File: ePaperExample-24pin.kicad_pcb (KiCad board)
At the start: 2 copper layers, 20 parts, among them J1 Conn_01x24_MountingPin, Q1 Q_NMOS_GSD

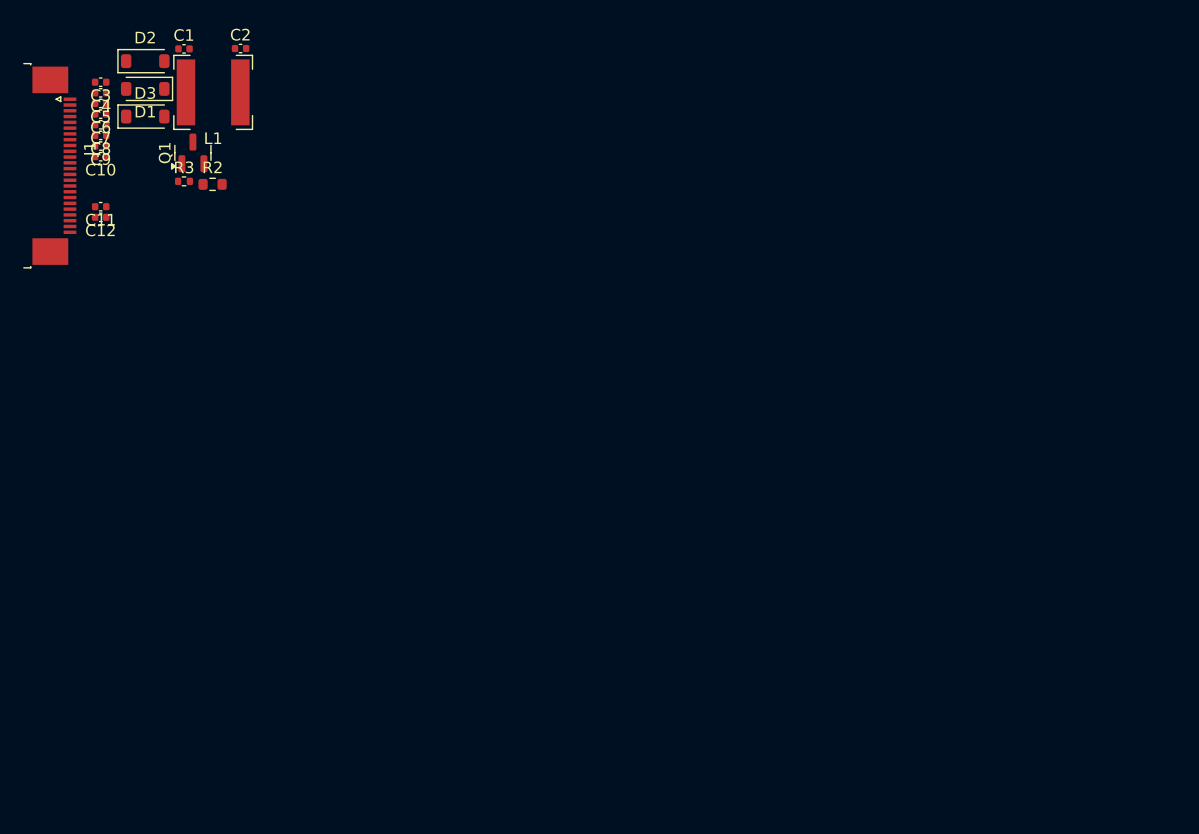
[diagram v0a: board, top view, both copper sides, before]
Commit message: Added updated schematic, added PCB layout
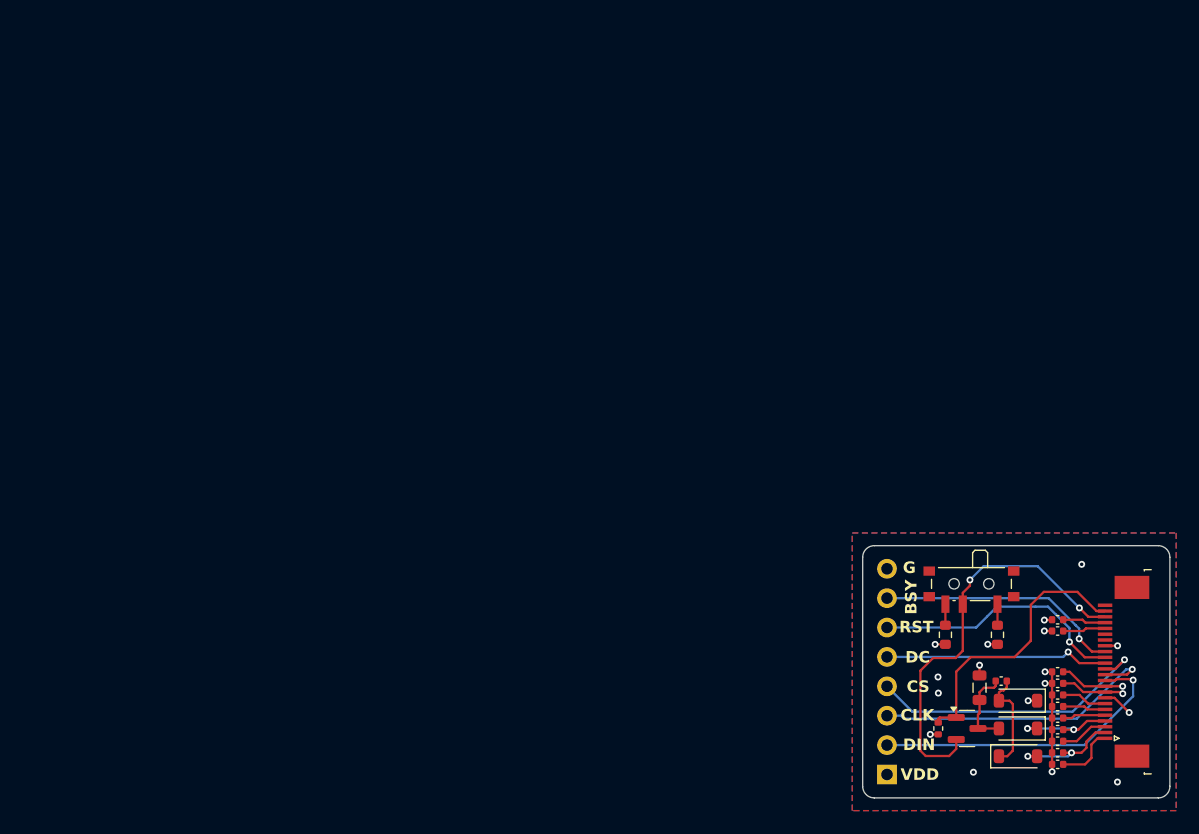
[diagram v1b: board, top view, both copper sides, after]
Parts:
- added J2: Conn_01x08_Socket, Connector_PinHeader_2.54mm:PinHeader_1x08_P2.54mm_Vertical, B.Cu at (129.0, 111.5)
- added R1: 1MR, Resistor_SMD:R_0402_1005Metric, F.Cu at (133.4, 107.5)
- added SW1: SW_SPDT, Button_Switch_SMD:SW_SPDT_PCM12, F.Cu at (136.3, 95.3)
- C1: value 100nF -> 1uF
- C2: value 4.7uF -> 1uF
- C4, C9: value 1uF -> 4.7uF
- L1: value 68uH -> 10uH; footprint Inductor_SMD:L_Bourns-SRN6028 -> Inductor_SMD:L_0805_2012Metric
- R2: value 3R -> 0R47
- R3: value 1MR -> 3R; footprint Resistor_SMD:R_0402_1005Metric -> Resistor_SMD:R_0603_1608Metric
- moved J1 102.0 mm to (149.2, 102.6), turned to 90 degrees
- moved C3 100.4 mm to (143.8, 108.6), turned to 0 degrees
- moved C5 98.8 mm to (143.8, 107.6), turned to 0 degrees
- moved C6 97.8 mm to (143.8, 106.6), turned to 0 degrees
- moved C1 97.6 mm to (143.8, 110.6)
- moved C7 96.8 mm to (143.8, 105.6), turned to 0 degrees
- moved C8 95.8 mm to (143.8, 104.6), turned to 0 degrees
- moved D1 95.0 mm to (140.3, 109.9), turned to 0 degrees
- moved D2 95.0 mm to (140.3, 107.5), turned to 180 degrees
- moved C9 94.9 mm to (143.8, 103.6), turned to 0 degrees
- moved C10 93.9 mm to (143.8, 102.6), turned to 0 degrees
- moved C2 93.2 mm to (143.8, 109.6)
- moved C4 93.0 mm to (138.9, 103.4)
- moved D3 90.8 mm to (140.3, 105.1), turned to 180 degrees
- moved C11 90.5 mm to (143.8, 99.1), turned to 0 degrees
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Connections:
- C1 pad 1: Net-(D1-K) -> GND
- C1 pad 2: Net-(D3-A) -> /VCOM
- C10 pad 2: +3.3V -> VDD
- C2 pad 2: +3.3V -> /PREVGL
- C3 pad 2: /VCOM -> /VSL
- C4 pad 1: GND -> Net-(D1-K)
- C4 pad 2: /PREVGL -> Net-(D2-A)
- C5 pad 2: /VSL -> /PREVGH
- C6 pad 2: /PREVGH -> /VSH
- C7 pad 2: /VSH -> /VPP
- C8 pad 2: /VPP -> Net-(J1-Pin_7)
- C9 pad 2: /VDD -> VDD
- D2 pad 1: GND -> /PREVGH
- D2 pad 2: Net-(D1-K) -> Net-(D2-A)
- D3 pad 1: /PREVGH -> GND
- D3 pad 2: Net-(D3-A) -> Net-(D1-K)
- J1 pad 10: +3.3V -> VDD
- J1 pad 17: /BS -> GND
- J1 pad 7: /VDD -> Net-(J1-Pin_7)
- J1 pad 9: +3.3V -> VDD
- L1 pad 1: Net-(D3-A) -> Net-(D2-A)
- L1 pad 2: +3.3V -> VDD
- Q1 pad 2: Net-(Q1-S) -> /RESE
- Q1 pad 3: Net-(D3-A) -> Net-(D2-A)
- R2 pad 1: Net-(Q1-S) -> Net-(SW1-C)
- R3 pad 1: /GDR -> Net-(SW1-A)
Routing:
- net VDD: track 0.00 -> 42.1 mm, vias 0 -> 3
- net /RESE: track 0.00 -> 36.0 mm, vias 0 -> 2
- net /DIN: track 0.00 -> 26.9 mm, vias 0 -> 1
- net /CLK: track 0.00 -> 25.6 mm, vias 0 -> 1
- net /EPD_CS: track 0.00 -> 25.3 mm, vias 0 -> 1
- net /GDR: track 0.00 -> 24.1 mm
- net /EPD_RST: track 0.00 -> 22.1 mm, vias 0 -> 1
- net /EPD_BUSY: track 0.00 -> 21.3 mm, vias 0 -> 1
- net /EPD_DC: track 0.00 -> 19.4 mm, vias 0 -> 1
- net GND: track 0.00 -> 18.1 mm, vias 0 -> 16
- net /PREVGL: track 0.00 -> 9.37 mm, vias 0 -> 2
- net Net-(D1-K): track 0.00 -> 8.86 mm
- net /PREVGH: track 0.00 -> 8.81 mm, vias 0 -> 2
- net Net-(D2-A): track 0.00 -> 7.06 mm
- net /VCOM: track 0.00 -> 5.24 mm
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- added copper zone on B.Cu, net GND
- added copper zone on F.Cu, net GND
- added copper zone on In1.Cu, net GND
- added copper zone on In2.Cu, net GND
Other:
- board outline added: 26.5 x 21.8 mm
- copper layers 2 -> 4
- board text added: "BSY"
- board text added: "CLK"
- board text added: "CS"
- board text added: "DC"
- board text added: "DIN"
- board text added: "G"
- board text added: "RST"
- board text added: "VDD"
